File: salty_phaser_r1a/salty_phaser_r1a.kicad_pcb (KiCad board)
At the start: 2 copper layers, 86.4 x 111.8 mm, 138 parts, among them X1 COM, X2 COM, X3 COM

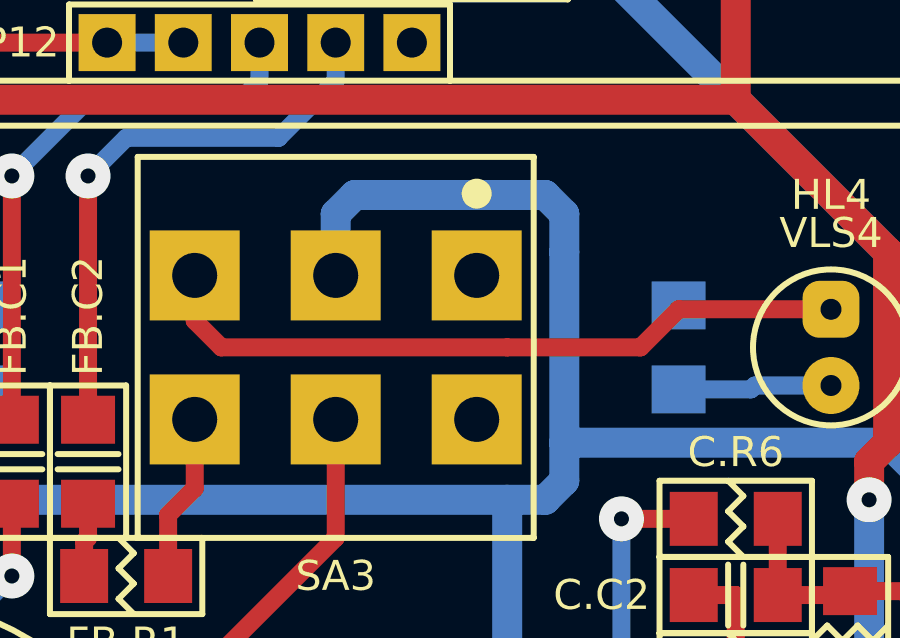
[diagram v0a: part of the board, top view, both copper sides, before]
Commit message: Salty Phaser [REV1]: minor changes
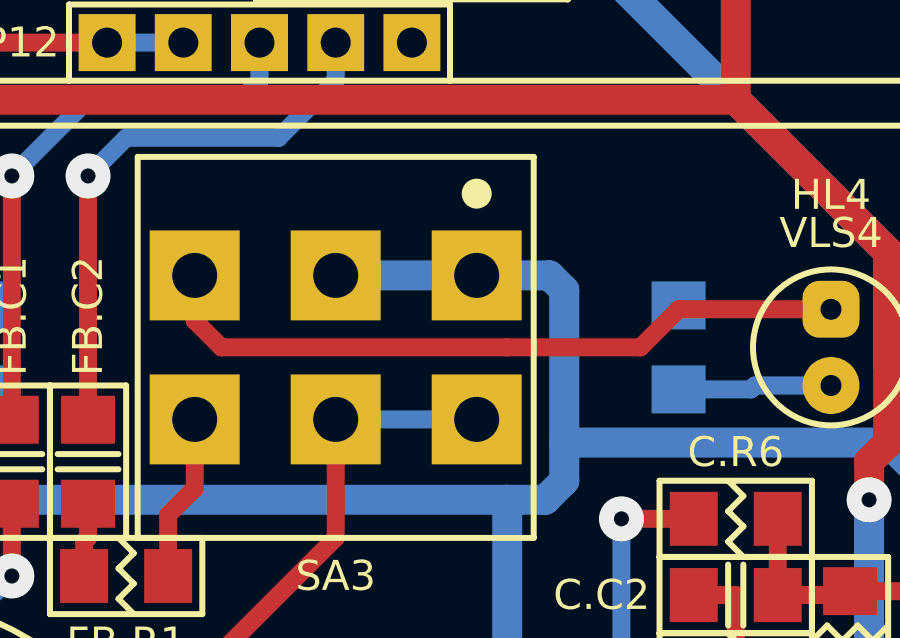
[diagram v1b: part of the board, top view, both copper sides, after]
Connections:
- SA3 pad NC1: Net-(SA3-PadNC1) -> V
- SA3 pad NC2: /FB-OFF -> /FB
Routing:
- net V: track 432.4 -> 427.4 mm
- net /FB: track 76.2 -> 80.9 mm

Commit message: Salty Phaser [REV1A]: 2.6 mm holes increased to 2.8 mm
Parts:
- RPB1: footprint SBKCL-TH-ML:RPB-18-3x17-PNL-7.4-2.6 -> SBKCL-TH-ML:RPB-1590BB-18-3x17-1.5-PNL-7.4-2.8
- RPB2: footprint SBKCL-TH-ML:RPB-18-2x17-PNL-7.4-2.6 -> SBKCL-TH-ML:RPB-1590BB-18-2x17-1.5-PNL-7.4-2.8

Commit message: Salty Phaser [REV1A]: many values changed based on debugging results
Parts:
- A.C1, A.C2, B.C1, B.C2, E.C1, E.C2, F.C1, F.C2: value 332 -> X
- A.D1, B.D1, E.D1, F.D1: value 13700 -> X
- A.R1, A.R4, A.R6, A.R9, B.R1, B.R4, B.R6, B.R9, E.R1, E.R4, E.R6, E.R9, F.R1, F.R4, F.R6, F.R9, FB.R1: value 273 -> X
- A.R10, A.R5, B.R10, B.R5, E.R10, E.R5, F.R10, F.R5, R2, R3, R4: value 103 -> X
- A.R2, A.R7, B.R2, B.R7, E.R2, E.R7, F.R2, F.R7: value 182 -> X
- A.R3, A.R8, B.R3, B.R8, E.R3, E.R8, F.R3, F.R8: value 203 -> X
- C.R3, C.R8, D.R3, D.R8: value 203 -> 103
- FB.C1, FB.C2: value 105 -> X
- HL2, HL3, HL4: value FYL-5013UWC -> X
- L.C1: value 475 -> 474
- L.C2: value 686 -> 475
- L.R2: value 683 -> 154
- MS.R2: value 620 -> 680
- MS.R3: value 111 -> 470
- OM.R1: value 154 -> X
- PS.R1, PS.R2: value 105 -> 103
- RPB1: value B100K-A1K-B100K -> B500K-A1K-B100K
- RPB2: value A50K-B100K -> X
- SA1: value RBS-1-2P6W-20VP -> X
- SA3: value MTS-202-A2 -> X
- VLS2, VLS3, VLS4: value BR-12.7 -> X
- X3: value COM -> X

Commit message: Minor changes
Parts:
- L.C2, PS.C3: footprint SBKCL:CP-RADIAL-D05.0-P02.0-CLS -> KCL-TH-SL:CP-RADIAL-D05.0-P02.0-CLS

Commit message: Salty Phaser [REV1A]: minor changes
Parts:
- IO.D1, L.D1: footprint KCL:P-SO-08 -> KCL-SM:P-SO-08
- PS.C1: footprint SBKCL:CP-RADIAL-D05.0-P02.0-CLS-OR-D06.3-P02.5-OR-D08.0-P03.5-CLS -> SBKCL-TH-SL:CP-RADIAL-D05.0-P02.0-CLS-OR-D06.3-P02.5-OR-D08.0-P03.5-CLS
- VLS1, VLS2, VLS3, VLS4: footprint KCL:VLS-BR -> KCL-VIRTUAL:VLS-BR
- X2, X3: footprint KCL:CON-PAD-S-1.0-1.9 -> KCL-TH-SL:CON-PAD-S-1.0-1.9
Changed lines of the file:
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@@
       (net 80 "Net-(IO.D1-Pad7)"))
   )
-  (module SBKCL:CP-RADIAL-D05.0-P02.0-CLS-OR-D06.3-P02.5-OR-D08.0-P03.5-CLS (layer F.Cu)
+  (module SBKCL-TH-SL:CP-RADIAL-D05.0-P02.0-CLS-OR-D06.3-P02.5-OR-D08.0-P03.5-CLS (layer F.Cu)
     (at 134.62 104.14)
     (fp_text reference PS.C1 (at 0.635 5.08) (layer F.SilkS)
@@
       (net 13 /LFO-AUTO))
   )
-  (module KCL:CON-PAD-S-1.0-1.9 (layer F.Cu)
+  (module KCL-TH-SL:CON-PAD-S-1.0-1.9 (layer F.Cu)
     (at 106.68 134.62)
     (fp_text reference X3 (at 0 -1.5875) (layer F.SilkS)
@@
       (net 1 COM))
   )
-  (module KCL:CON-PAD-S-1.0-1.9 (layer F.Cu)
+  (module KCL-TH-SL:CON-PAD-S-1.0-1.9 (layer F.Cu)
     (at 104.14 134.62)
     (fp_text reference X2 (at 0 -1.5875) (layer F.SilkS)
@@
       (net 3 /LED))
   )
-  (module KCL:VLS-BR (layer F.Cu)
+  (module KCL-VIRTUAL:VLS-BR (layer F.Cu)
     (at 138.43 138.43)
     (fp_text reference VLS4 (at 0 -3.81) (layer F.SilkS)
@@
     (fp_circle (center 0 0) (end 2.6 0) (layer F.CrtYd) (width 0.1))
   )
-  (module KCL:VLS-BR (layer F.Cu)
+  (module KCL-VIRTUAL:VLS-BR (layer F.Cu)
     (at 105.41 138.43)
     (fp_text reference VLS3 (at 0 5.08) (layer F.SilkS)
@@
     (fp_circle (center 0 0) (end 2.6 0) (layer F.CrtYd) (width 0.1))
   )
-  (module KCL:VLS-BR (layer F.Cu)
+  (module KCL-VIRTUAL:VLS-BR (layer F.Cu)
     (at 72.39 138.43)
     (fp_text reference VLS2 (at 0 -3.81) (layer F.SilkS)
@@
       (net 11 /OUT10))
   )
-  (module KCL:P-SO-08 (layer B.Cu)
+  (module KCL-SM:P-SO-08 (layer B.Cu)
     (at 106.68 184.785)
     (fp_text reference IO.D1 (at 0 3.4925) (layer B.SilkS)
@@
       (net 6 /DRY))
   )
-  (module KCL:P-SO-08 (layer F.Cu)
+  (module KCL-SM:P-SO-08 (layer F.Cu)
     (at 105.41 118.745 180)
     (fp_text reference L.D1 (at 0 -3.4925) (layer F.SilkS)
@@
       (net 11 /OUT10))
   )
-  (module KCL:VLS-BR (layer F.Cu)
+  (module KCL-VIRTUAL:VLS-BR (layer F.Cu)
     (at 105.41 179.07)
     (fp_text reference VLS1 (at 0 3.81) (layer F.SilkS)

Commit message: Salty Phaser [REV1A]: minor changes
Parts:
- SA2, SA3: footprint KCL-TH-ML:SW-MTS-202-A2-PNL-6.0 -> KCL-TH-ML:SW-MTS-202-A2-3.0-PNL-6.0
- VMH1, VMH2, VMH3, VMH4, VMH5, VMH6: footprint KCL:VMH-STA-DA5 -> KCL-TH-ML:VMH-STA-DA5-PNL-3.0

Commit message: Salty Phaser [REV1A]: minor changes
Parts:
- A.C1, A.C2, B.C1, B.C2, C.C1, C.C2, D.C1, D.C2, E.C1, E.C2, F.C1, F.C2, FB.C1, FB.C2, IB.C1, L.C1, OM.C1, PS.C2: footprint KCL:C-SM-1206 -> KCL-SM:C-SM-1206
- A.D1, B.D1, C.D1, D.D1, E.D1, F.D1: footprint KCL:P-SO-16 -> KCL-SM:P-SO-16
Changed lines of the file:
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@@
       (net 34 "Net-(SA1-Pad2-1)"))
   )
-  (module KCL:C-SM-1206 (layer F.Cu)
+  (module KCL-SM:C-SM-1206 (layer F.Cu)
     (at 114.3 107.95 90)
     (fp_text reference PS.C2 (at 0 2.2225 90) (layer F.SilkS)
@@
       (net 1 COM))
   )
-  (module KCL:C-SM-1206 (layer F.Cu)
+  (module KCL-SM:C-SM-1206 (layer F.Cu)
     (at 135.255 146.685 180)
     (fp_text reference C.C2 (at 2.8575 0) (layer F.SilkS)
@@
       (net 55 "Net-(C.D1-Pad4)"))
   )
-  (module KCL:P-SO-16 (layer F.Cu)
+  (module KCL-SM:P-SO-16 (layer F.Cu)
     (at 135.89 156.845 180)
     (fp_text reference C.D1 (at -5.08 0 270) (layer F.SilkS)
@@
       (net 20 /LFO))
   )
-  (module KCL:C-SM-1206 (layer F.Cu)
+  (module KCL-SM:C-SM-1206 (layer F.Cu)
     (at 146.05 153.67 90)
     (fp_text reference C.C1 (at 2.8575 0 270) (layer F.SilkS)
@@
       (net 95 "Net-(D.C2-Pad1)"))
   )
-  (module KCL:C-SM-1206 (layer F.Cu)
+  (module KCL-SM:C-SM-1206 (layer F.Cu)
     (at 75.565 167.005)
     (fp_text reference D.C2 (at 2.8575 0) (layer F.SilkS)
@@
       (net 61 "Net-(D.D1-Pad4)"))
   )
-  (module KCL:P-SO-16 (layer F.Cu)
+  (module KCL-SM:P-SO-16 (layer F.Cu)
     (at 74.93 156.845)
     (fp_text reference D.D1 (at -5.08 0 90) (layer F.SilkS)
@@
       (net 64 "Net-(D.D1-Pad16)"))
   )
-  (module KCL:C-SM-1206 (layer F.Cu)
+  (module KCL-SM:C-SM-1206 (layer F.Cu)
     (at 64.77 160.02 270)
     (fp_text reference D.C1 (at 2.8575 0 270) (layer F.SilkS)
@@
       (net 10 /OUT8))
   )
-  (module KCL:C-SM-1206 (layer F.Cu)
+  (module KCL-SM:C-SM-1206 (layer F.Cu)
     (at 77.47 194.31)
     (fp_text reference E.C2 (at 0 2.2225) (layer F.SilkS)
@@
       (net 1 COM))
   )
-  (module KCL:C-SM-1206 (layer F.Cu)
+  (module KCL-SM:C-SM-1206 (layer F.Cu)
     (at 69.85 184.15 270)
     (fp_text reference E.C1 (at -2.8575 0 270) (layer F.SilkS)
@@
       (net 49 "Net-(B.D1-Pad4)"))
   )
-  (module KCL:C-SM-1206 (layer F.Cu)
+  (module KCL-SM:C-SM-1206 (layer F.Cu)
     (at 128.27 194.31)
     (fp_text reference B.C2 (at 0 2.2225) (layer F.SilkS)
@@
       (net 1 COM))
   )
-  (module KCL:C-SM-1206 (layer F.Cu)
+  (module KCL-SM:C-SM-1206 (layer F.Cu)
     (at 120.65 184.15 270)
     (fp_text reference B.C1 (at -2.8575 0 270) (layer F.SilkS)
@@
       (net 7 /OUT2))
   )
-  (module KCL:C-SM-1206 (layer B.Cu)
+  (module KCL-SM:C-SM-1206 (layer B.Cu)
     (at 140.97 184.15 270)
     (fp_text reference A.C1 (at -4.1275 0 90) (layer B.SilkS)
@@
       (net 46 "Net-(A.D1-Pad16)"))
   )
-  (module KCL:C-SM-1206 (layer B.Cu)
+  (module KCL-SM:C-SM-1206 (layer B.Cu)
     (at 133.35 194.31 180)
     (fp_text reference A.C2 (at 0 -2.2225) (layer B.SilkS)
@@
       (net 101 "Net-(L.D1-Pad1)"))
   )
-  (module KCL:P-SO-16 (layer B.Cu)
+  (module KCL-SM:P-SO-16 (layer B.Cu)
     (at 80.01 186.055 180)
     (fp_text reference F.D1 (at 0 6.0325) (layer B.SilkS)
@@
       (net 16 /OUT12))
   )
-  (module KCL:P-SO-16 (layer F.Cu)
+  (module KCL-SM:P-SO-16 (layer F.Cu)
     (at 80.01 186.055)
     (fp_text reference E.D1 (at 0 -6.0325) (layer F.SilkS)
@@
       (net 11 /OUT10))
   )
-  (module KCL:P-SO-16 (layer F.Cu)
+  (module KCL-SM:P-SO-16 (layer F.Cu)
     (at 130.81 186.055)
     (fp_text reference B.D1 (at 0 -6.0325) (layer F.SilkS)
@@
       (net 8 /OUT4))
   )
-  (module KCL:P-SO-16 (layer B.Cu)
+  (module KCL-SM:P-SO-16 (layer B.Cu)
     (at 130.81 186.055 180)
     (fp_text reference A.D1 (at 0 6.0325) (layer B.SilkS)
@@
       (net 42 "Net-(A.D1-Pad1)"))
   )
-  (module KCL:C-SM-1206 (layer F.Cu)
+  (module KCL-SM:C-SM-1206 (layer F.Cu)
     (at 104.14 185.42 180)
     (fp_text reference OM.C1 (at -2.8575 0) (layer F.SilkS)
@@
       (net 80 "Net-(IO.D1-Pad7)"))
   )
-  (module KCL:C-SM-1206 (layer B.Cu)
+  (module KCL-SM:C-SM-1206 (layer B.Cu)
     (at 97.79 182.88)
     (fp_text reference IB.C1 (at -0.9525 4.7625) (layer B.SilkS)
@@
       (net 86 "Net-(IB.C1-Pad2)"))
   )
-  (module KCL:C-SM-1206 (layer F.Cu)
+  (module KCL-SM:C-SM-1206 (layer F.Cu)
     (at 114.3 113.03 270)
     (fp_text reference L.C1 (at 0 -2.2225 90) (layer F.SilkS)
@@
       (net 1 COM))
   )
-  (module KCL:C-SM-1206 (layer F.Cu)
+  (module KCL-SM:C-SM-1206 (layer F.Cu)
     (at 113.665 142.24 270)
     (fp_text reference FB.C2 (at -2.8575 0 90) (layer F.SilkS)
@@
       (net 37 "Net-(FB.C2-Pad1)"))
   )
-  (module KCL:C-SM-1206 (layer F.Cu)
+  (module KCL-SM:C-SM-1206 (layer F.Cu)
     (at 111.125 142.24 90)
     (fp_text reference FB.C1 (at 2.8575 0 270) (layer F.SilkS)
@@
       (net 12 /WET))
   )
-  (module KCL:C-SM-1206 (layer B.Cu)
+  (module KCL-SM:C-SM-1206 (layer B.Cu)
     (at 82.55 194.31 180)
     (fp_text reference F.C2 (at 0 -2.2225) (layer B.SilkS)
@@
       (net 73 "Net-(F.C2-Pad1)"))
   )
-  (module KCL:C-SM-1206 (layer B.Cu)
+  (module KCL-SM:C-SM-1206 (layer B.Cu)
     (at 90.17 184.15 270)
     (fp_text reference F.C1 (at -4.1275 0 90) (layer B.SilkS)
